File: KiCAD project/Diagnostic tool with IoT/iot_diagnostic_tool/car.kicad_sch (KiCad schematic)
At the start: 17 parts, among them Q1 s8050, Q2 s8050, U3 SN65HVD231

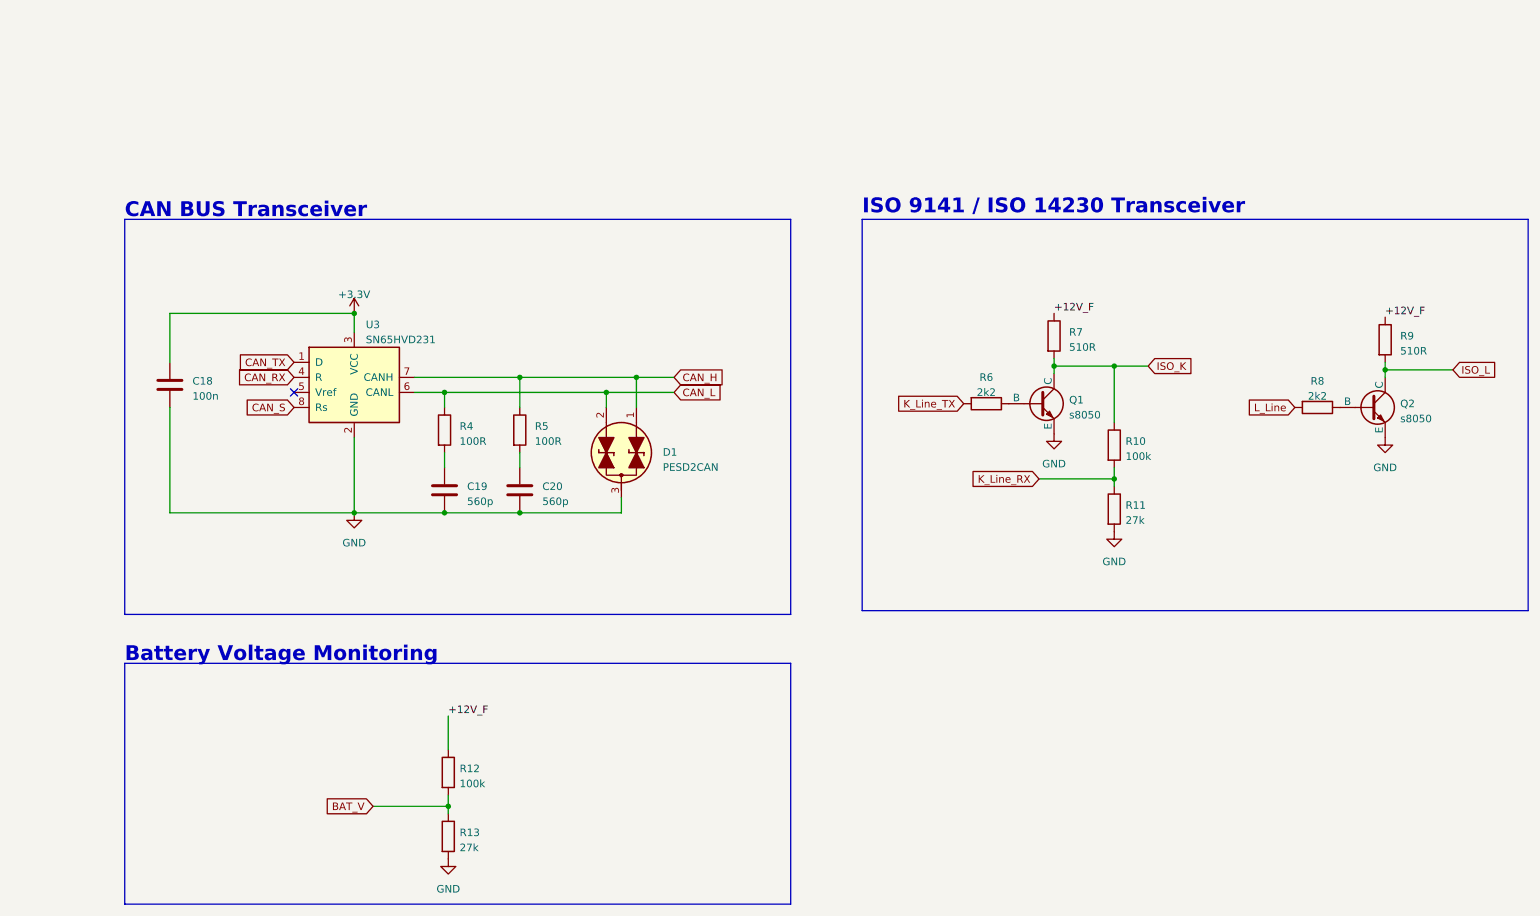
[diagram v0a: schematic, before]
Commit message: Update 03/03/23 - new schematic done
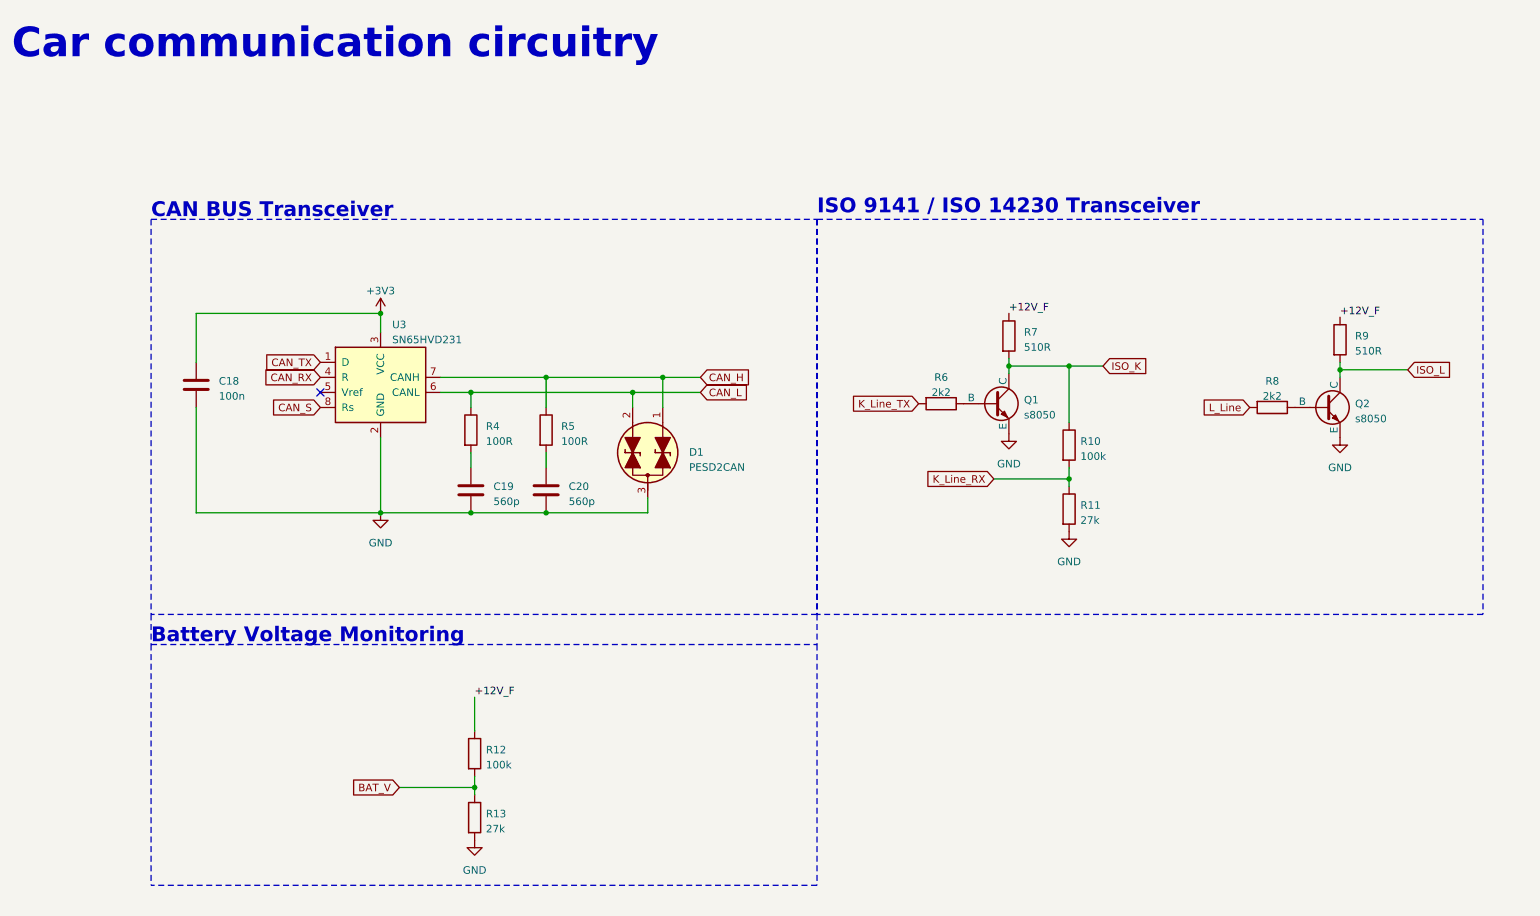
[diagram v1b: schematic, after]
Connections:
- net +3.3V renamed +3V3
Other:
- note added: "Car communication circuitry"
- moved on the sheet: C18, C19, C20, D1, Q1, Q2, R10, R11, R12, R13, R4, R5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

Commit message: Update 06/03/23 - new board layout WIP 70%
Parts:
- C18: footprint (none) -> Capacitor_SMD:C_0402_1005Metric
- C19, C20: footprint (none) -> Capacitor_SMD:C_0402_1005Metric_Pad0.74x0.62mm_HandSolder
- D1: footprint Package_TO_SOT_SMD_AKL:SOT-23 -> Package_TO_SOT_SMD:SOT-23
- Q1, Q2: footprint (none) -> Package_TO_SOT_SMD:SOT-23
- R10, R11, R12, R13, R4, R5, R6, R7, R8, R9: footprint (none) -> Resistor_SMD:R_0402_1005Metric
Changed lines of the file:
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@@
       (effects (font (size 1.27 1.27)) (justify left))
     )
-    (property "Footprint" "" (at 88.392 146.685 90)
+    (property "Footprint" "Resistor_SMD:R_0402_1005Metric" (at 88.392 146.685 90)
       (effects (font (size 1.27 1.27)) hide)
     )
@@
       (effects (font (size 1.27 1.27)) (justify right))
     )
-    (property "Footprint" "Package_TO_SOT_SMD_AKL:SOT-23" (at 110.49 85.09 0)
+    (property "Footprint" "Package_TO_SOT_SMD:SOT-23" (at 110.49 85.09 0)
       (effects (font (size 1.27 1.27)) hide)
     )
@@
       (effects (font (size 1.27 1.27)) (justify left))
     )
-    (property "Footprint" "" (at 188.722 94.615 90)
+    (property "Footprint" "Resistor_SMD:R_0402_1005Metric" (at 188.722 94.615 90)
       (effects (font (size 1.27 1.27)) hide)
     )
@@
       (effects (font (size 1.27 1.27)) (justify left))
     )
-    (property "Footprint" "" (at 90.5002 95.25 0)
+    (property "Footprint" "Capacitor_SMD:C_0402_1005Metric_Pad0.74x0.62mm_HandSolder" (at 90.5002 95.25 0)
       (effects (font (size 1.27 1.27)) hide)
     )
@@
       (effects (font (size 1.27 1.27)) (justify left))
     )
-    (property "Footprint" "" (at 188.722 83.82 90)
+    (property "Footprint" "Resistor_SMD:R_0402_1005Metric" (at 188.722 83.82 90)
       (effects (font (size 1.27 1.27)) hide)
     )
@@
       (effects (font (size 1.27 1.27)))
     )
-    (property "Footprint" "" (at 168.91 75.057 90)
+    (property "Footprint" "Resistor_SMD:R_0402_1005Metric" (at 168.91 75.057 90)
       (effects (font (size 1.27 1.27)) hide)
     )
@@
       (effects (font (size 1.27 1.27)) (justify left))
     )
-    (property "Footprint" "" (at 88.392 135.89 90)
+    (property "Footprint" "Resistor_SMD:R_0402_1005Metric" (at 88.392 135.89 90)
       (effects (font (size 1.27 1.27)) hide)
     )
@@
       (effects (font (size 1.27 1.27)) (justify left))
     )
-    (property "Footprint" "" (at 234.442 66.04 90)
+    (property "Footprint" "Resistor_SMD:R_0402_1005Metric" (at 234.442 66.04 90)
       (effects (font (size 1.27 1.27)) hide)
     )
@@
       (effects (font (size 1.27 1.27)) (justify left))
     )
-    (property "Footprint" "" (at 241.3 76.835 0)
+    (property "Footprint" "Package_TO_SOT_SMD:SOT-23" (at 241.3 76.835 0)
       (effects (font (size 1.27 1.27)) hide)
     )
@@
       (effects (font (size 1.27 1.27)))
     )
-    (property "Footprint" "" (at 224.79 75.692 90)
+    (property "Footprint" "Resistor_SMD:R_0402_1005Metric" (at 224.79 75.692 90)
       (effects (font (size 1.27 1.27)) hide)
     )
@@
       (effects (font (size 1.27 1.27)) (justify left))
     )
-    (property "Footprint" "" (at 297.18 77.47 0)
+    (property "Footprint" "Package_TO_SOT_SMD:SOT-23" (at 297.18 77.47 0)
       (effects (font (size 1.27 1.27)) hide)
     )
@@
       (effects (font (size 1.27 1.27)) (justify left))
     )
-    (property "Footprint" "" (at 87.757 81.28 90)
+    (property "Footprint" "Resistor_SMD:R_0402_1005Metric" (at 87.757 81.28 90)
       (effects (font (size 1.27 1.27)) hide)
     )
@@
       (effects (font (size 1.27 1.27)) (justify left))
     )
-    (property "Footprint" "" (at 100.457 81.28 90)
+    (property "Footprint" "Resistor_SMD:R_0402_1005Metric" (at 100.457 81.28 90)
       (effects (font (size 1.27 1.27)) hide)
     )
@@
       (effects (font (size 1.27 1.27)) (justify left))
     )
-    (property "Footprint" "" (at 178.562 65.405 90)
+    (property "Footprint" "Resistor_SMD:R_0402_1005Metric" (at 178.562 65.405 90)
       (effects (font (size 1.27 1.27)) hide)
     )
@@
       (effects (font (size 1.27 1.27)) (justify left))
     )
-    (property "Footprint" "" (at 44.1452 77.47 0)
+    (property "Footprint" "Capacitor_SMD:C_0402_1005Metric" (at 44.1452 77.47 0)
       (effects (font (size 1.27 1.27)) hide)
     )
@@
       (effects (font (size 1.27 1.27)) (justify left))
     )
-    (property "Footprint" "" (at 103.2002 95.25 0)
-      (effects (font (size 1.27 1.27)) hide)
-    )
+    (property "Footprint" "Capacitor_SMD:C_0402_1005Metric_Pad0.74x0.62mm_HandSolder" (at 103.2002 95.25 0)
+      (effects (font (size 1.27 1.27)) hide)
+    )
